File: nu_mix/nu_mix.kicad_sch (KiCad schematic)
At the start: 61 parts, among them J1 2X5, J2 I/O connector, J3 I/O connector, Q1 LBSS84LT1G, SW1 SW_Slide_DP3T, SW2 SW_Slide_DP3T, SW3 SW_Slide_DP3T, SW4 SW_Slide_DP3T, SW5 SW_Slide_DP3T, SW6 SW_Slide_DP3T, SW7 SW_Slide_DP3T, SW8 SW_Slide_DP3T, U1 OPA202IDBVR, U2 OPA1692IDR

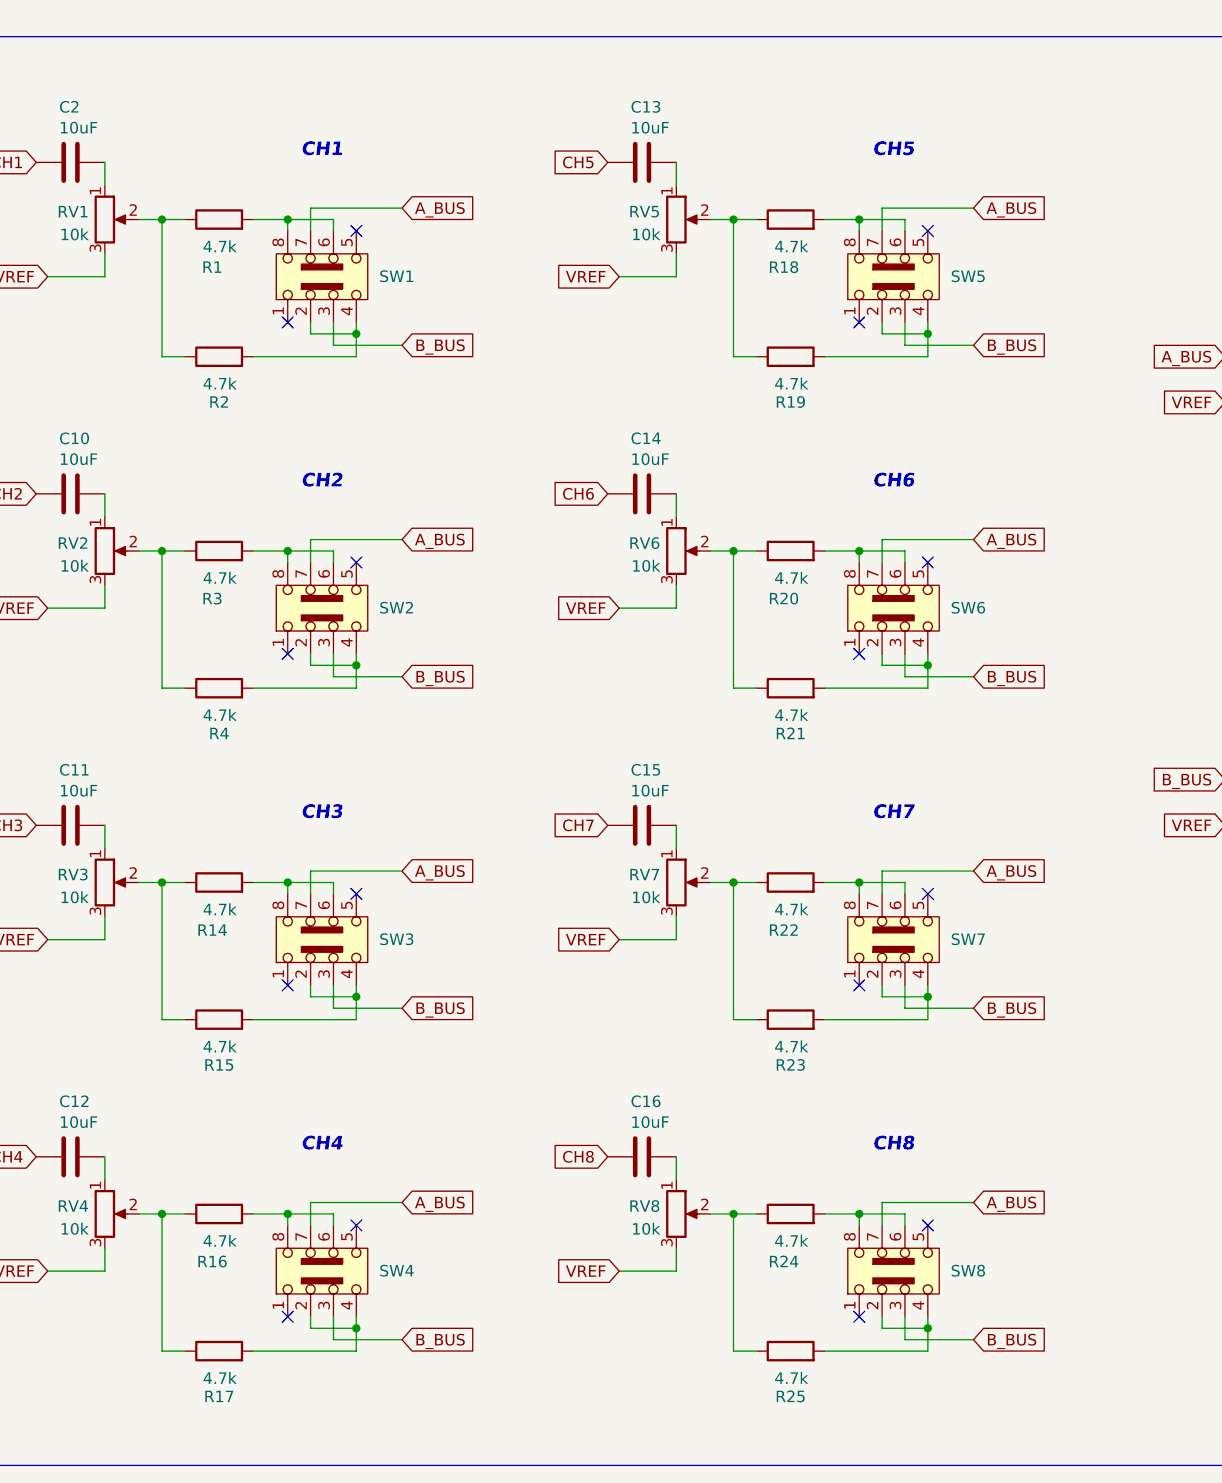
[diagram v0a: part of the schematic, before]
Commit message: Full layout
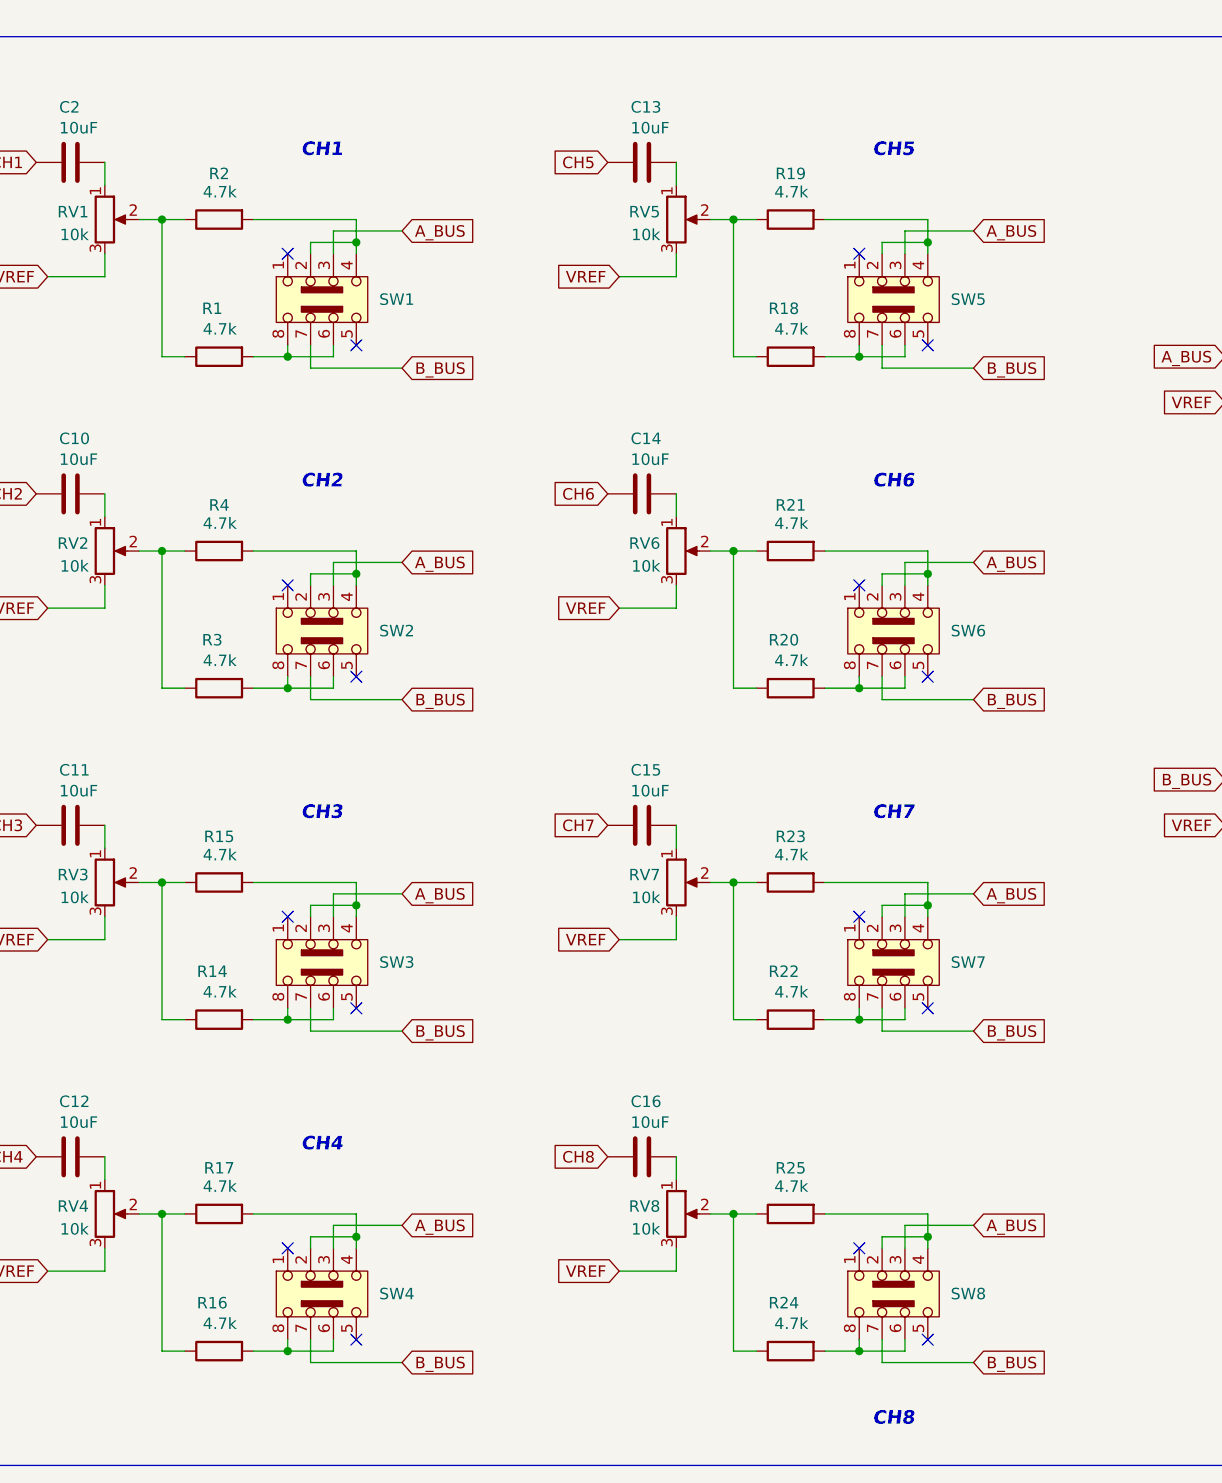
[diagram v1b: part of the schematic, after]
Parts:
- J1: footprint Connector_PinHeader_2.00mm:PinHeader_2x05_P2.00mm_Vertical -> cycfi_library:pin_header_2x5p_2.54mm_smd_horizontal
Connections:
- net A_BUS: now also SW1.3 (C1`), SW2.3 (C1`), SW3.3 (C1`), SW4.3 (C1`), SW5.3 (C1`), SW6.3 (C1`), SW7.3 (C1`), SW8.3 (C1`); no longer SW1.7 (C2), SW2.7 (C2), SW3.7 (C2), SW4.7 (C2), SW5.7 (C2), SW6.7 (C2), SW7.7 (C2), SW8.7 (C2)
- net B_BUS: now also SW1.7 (C2), SW2.7 (C2), SW3.7 (C2), SW4.7 (C2), SW5.7 (C2), SW6.7 (C2), SW7.7 (C2), SW8.7 (C2); no longer SW1.3 (C1`), SW2.3 (C1`), SW3.3 (C1`), SW4.3 (C1`), SW5.3 (C1`), SW6.3 (C1`), SW7.3 (C1`), SW8.3 (C1`)
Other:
- moved on the sheet: R1, R14, R15, R16, R17, R18, R19, R2, R20, R21, R22, R23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
